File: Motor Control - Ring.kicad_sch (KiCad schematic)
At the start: 9 parts, among them J5 BM09B-SRSS-TB, U13 TB9051FTG,EL

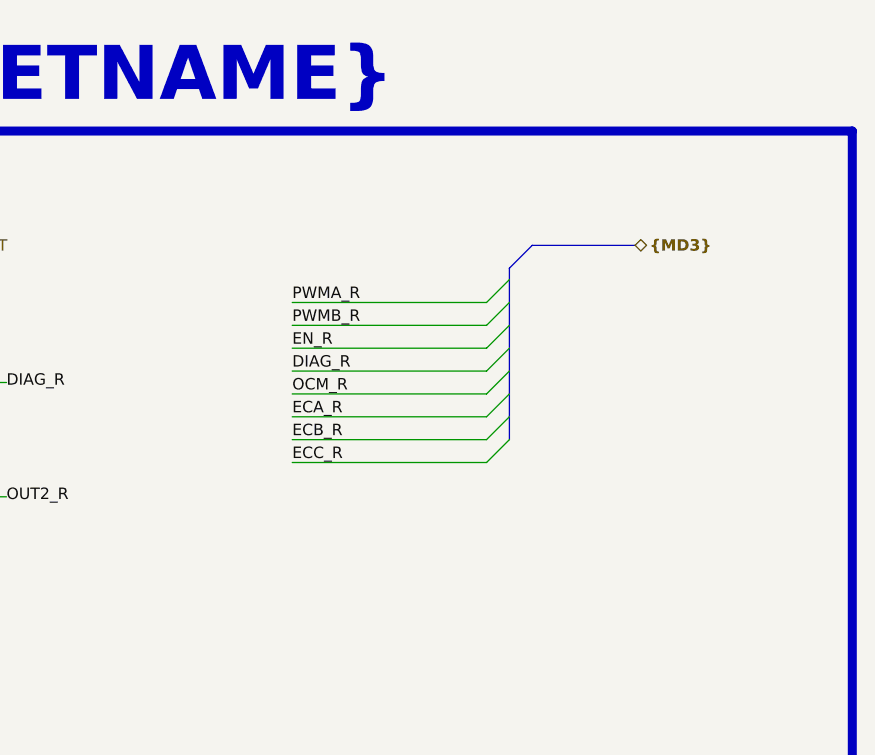
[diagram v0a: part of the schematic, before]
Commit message: Update Schematic
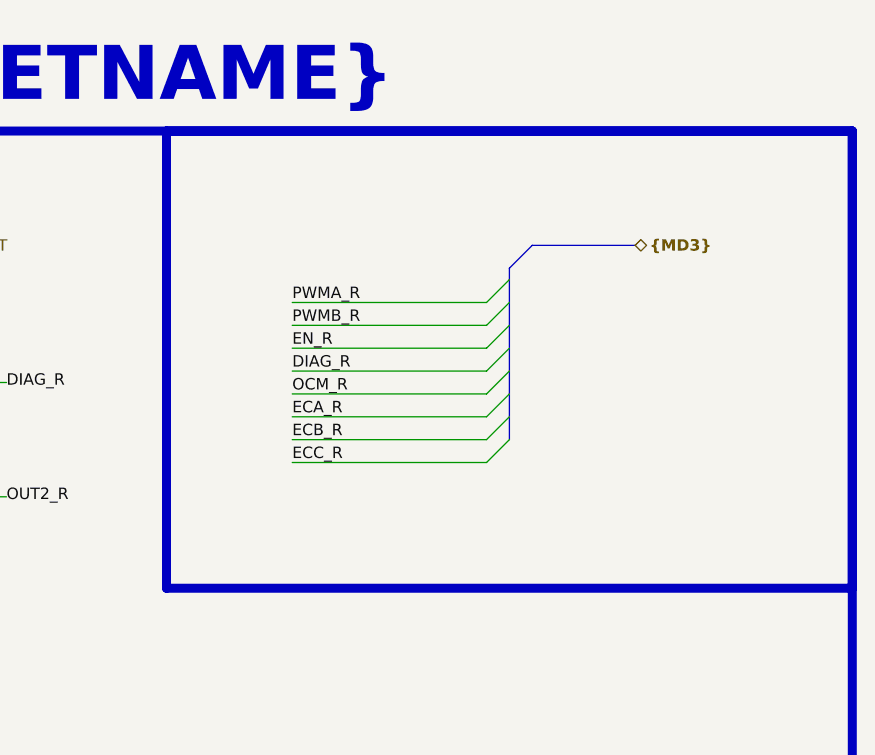
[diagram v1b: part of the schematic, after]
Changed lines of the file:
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@@
+	)
+	(rectangle
+		(start 177.8 25.4)
+		(end 254 76.2)
+		(stroke
+			(width 1)
+			(type default)
+			(color 200 0 0 1)
+		)
+		(fill
+			(type none)
+		)
 	)
 	(rectangle

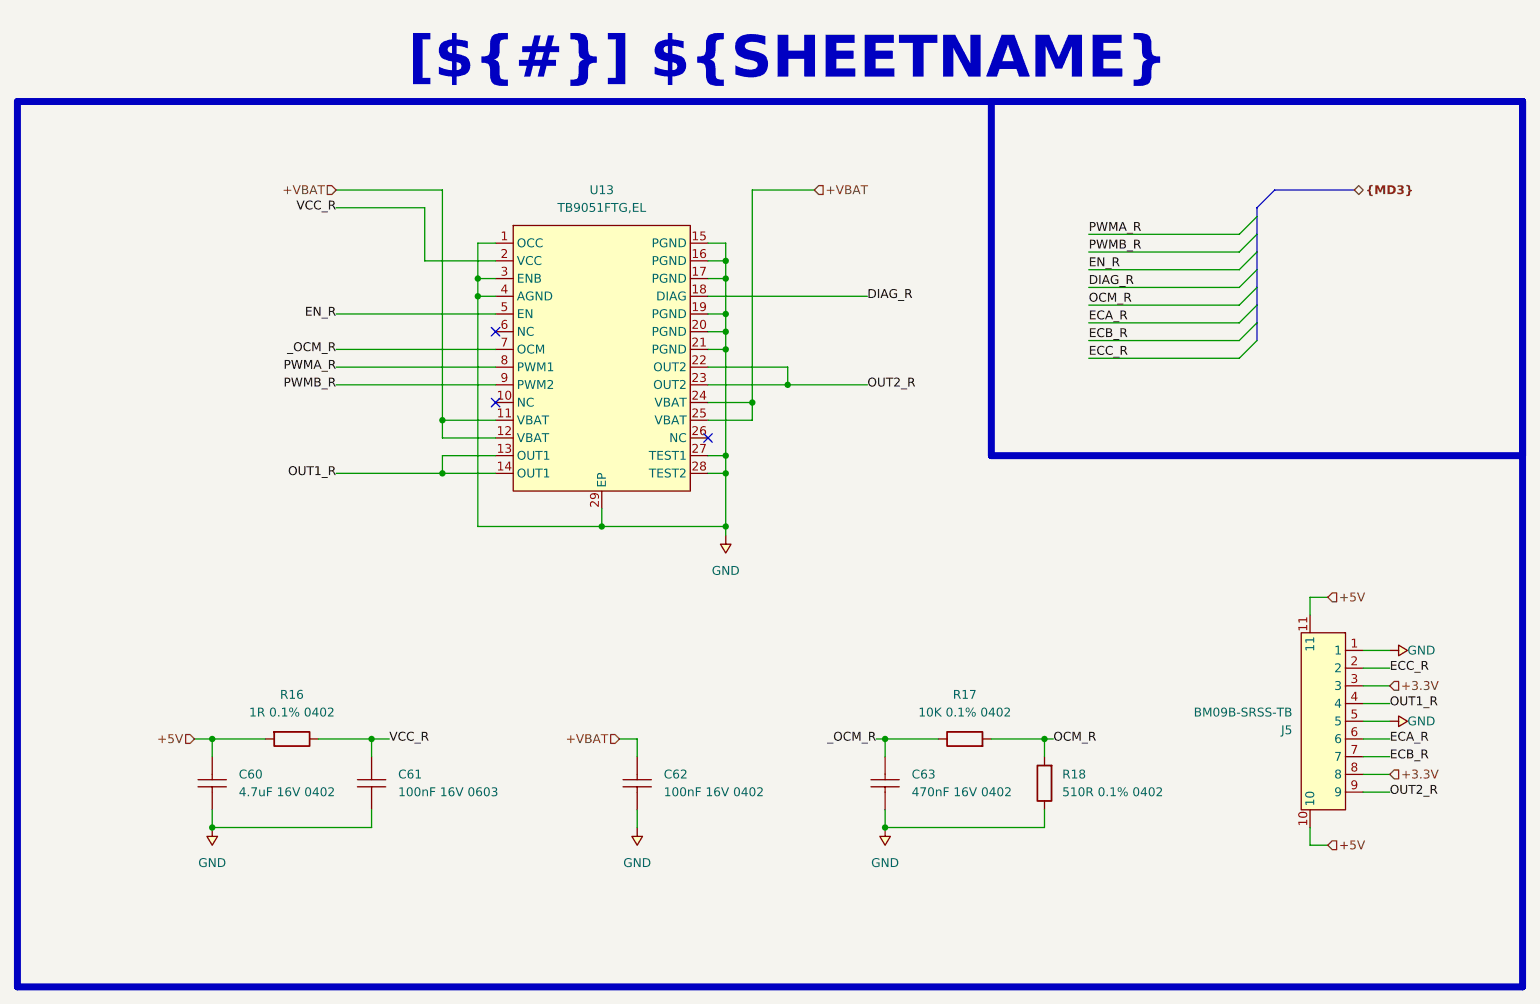
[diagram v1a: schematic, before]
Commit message: Update Schematic
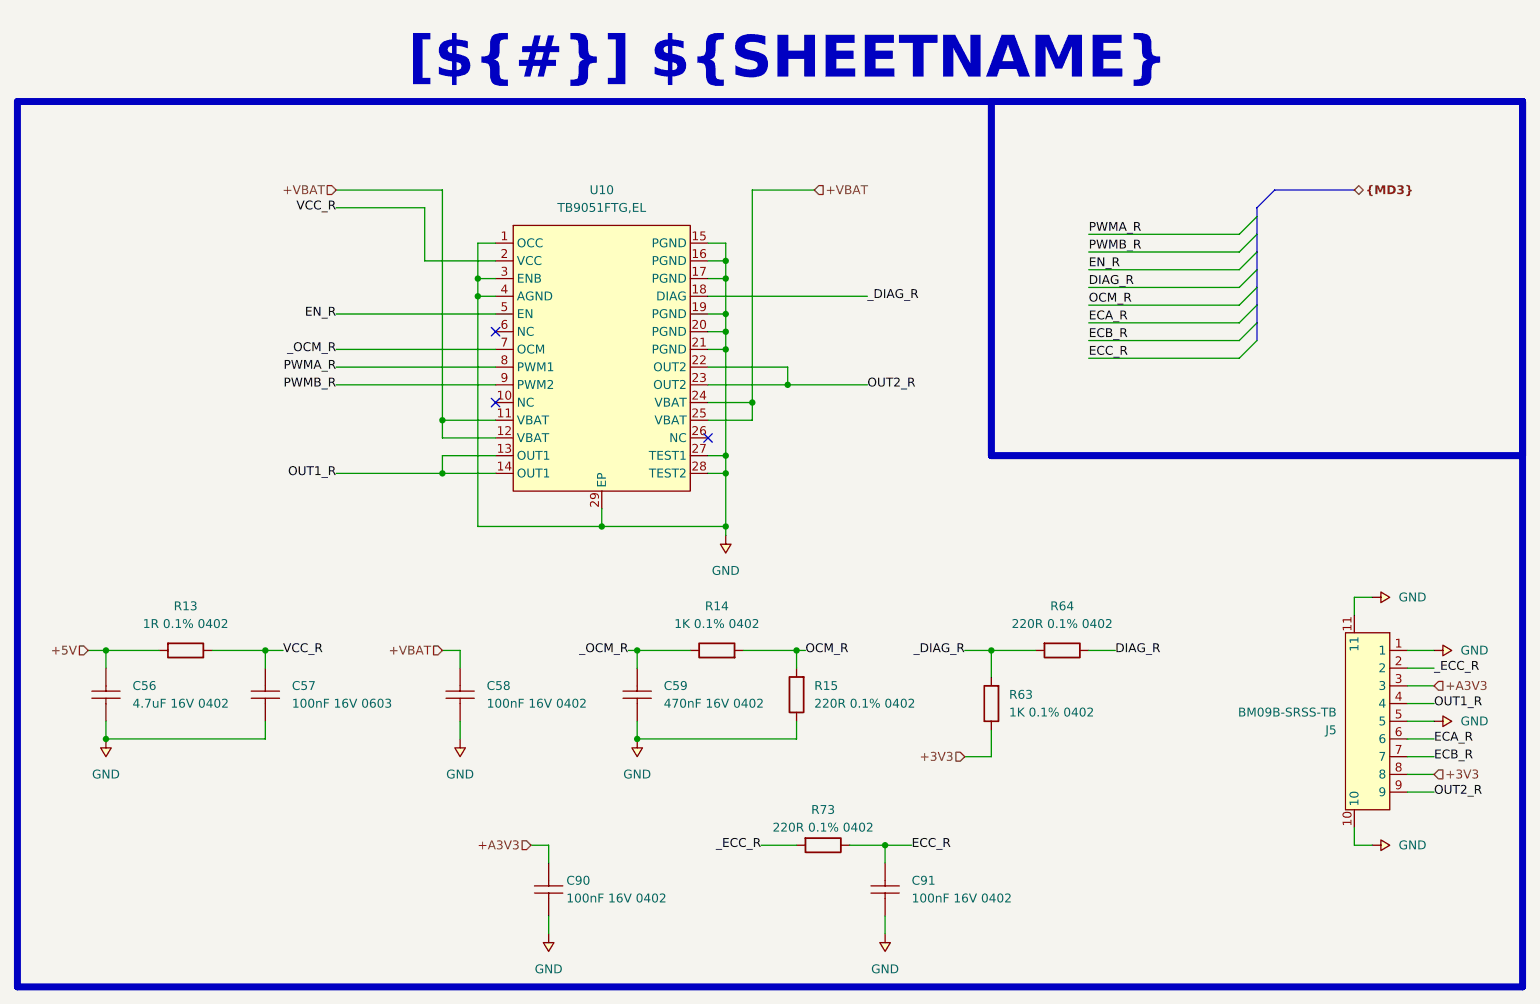
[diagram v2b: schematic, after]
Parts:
- added C90, C91: 100nF 16V 0402, Duc_Library:C0402, symbol Duc-Capacitors:CAP CER 0402
- added R63: 1K 0.1% 0402, Duc_Library:R0402, symbol Duc-Resistors:RES SMD 0402
- added R64, R73: 220R 0.1% 0402, Duc_Library:R0402, symbol Duc-Resistors:RES SMD 0402
- R14: renamed from R17; value 10K 0.1% 0402 -> 1K 0.1% 0402
- R15: renamed from R18; value 510R 0.1% 0402 -> 220R 0.1% 0402
- renumbered C60 to C56, C61 to C57, C62 to C58, C63 to C59, R16 to R13, U13 to U10
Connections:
- net +5V: no longer J5.10, J5.11
- net DIAG_R: now also R64.2; no longer U10.18 (DIAG)
- net ECC_R: now also C91.2, R73.2; no longer J5.2
- net GND: now also J5.10, J5.11, C90.1, C91.1
- net +3.3V renamed +3V3
- net +3V3: now also R63.2; no longer J5.3
- new net +A3V3: C90.2, J5.3
- new net _DIAG_R: R63.1, R64.1, U10.18 (DIAG)
- new net _ECC_R: J5.2, R73.1
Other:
- moved on the sheet: C56, C57, C58, C59, R13, R14, R15
